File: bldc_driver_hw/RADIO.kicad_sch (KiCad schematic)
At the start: 17 parts, among them SW2 SW_Push, SW3 SW_Push, U8 ESP32-C6-MINI-1

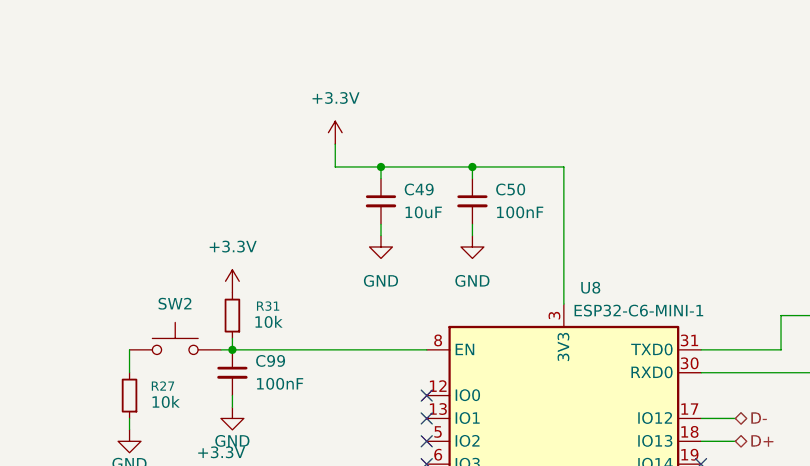
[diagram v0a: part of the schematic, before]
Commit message: board finished
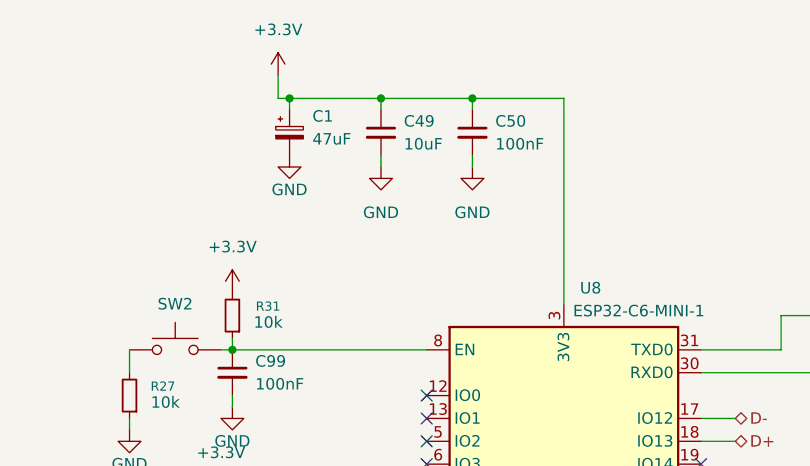
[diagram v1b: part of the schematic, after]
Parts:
- added C1: 47uF, Capacitor_Tantalum_SMD:CP_EIA-6032-15_Kemet-U, symbol Device:C_Polarized_Small
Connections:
- net +3.3V: now also C1.1
- net GND: now also C1.2
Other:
- moved on the sheet: C49, C50
